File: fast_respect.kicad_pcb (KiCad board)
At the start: 2 copper layers, 70 x 110 mm, 97 parts, among them J1_1 Conn_02x04_Odd_Even, J5_1 Conn_02x03_Odd_Even, J5_2 Conn_02x03_Odd_Even, J7_1 Conn_01x02, Q2_1 AONM7421, Q3_1 IRLML6344T, Q4_1 IRLML6344T, Q4_2 IRLML6344T, Q4_3 IRLML6344T, Q4_4 IRLML6344T, Q4_5 ST-1KL3A, Q4_6 ST-1KL3A, Q4_7 ST-1KL3A, Q4_8 ST-1KL3A, Q7_1 IRLML6344T, SW1_1 BOOT0_SW, SW1_2 NRST_SW, SW2_1 SW_SPDT, SW3_1 SW_Push, SW3_2 SW_Push, SW3_3 SW_Push, U1_1 STM32F446RETx, U2_1 AZ1117-5.0, U2_2 AZ1117-3.3, U5_1 DRV8835DSSR, U6_1 ICM-42688-P

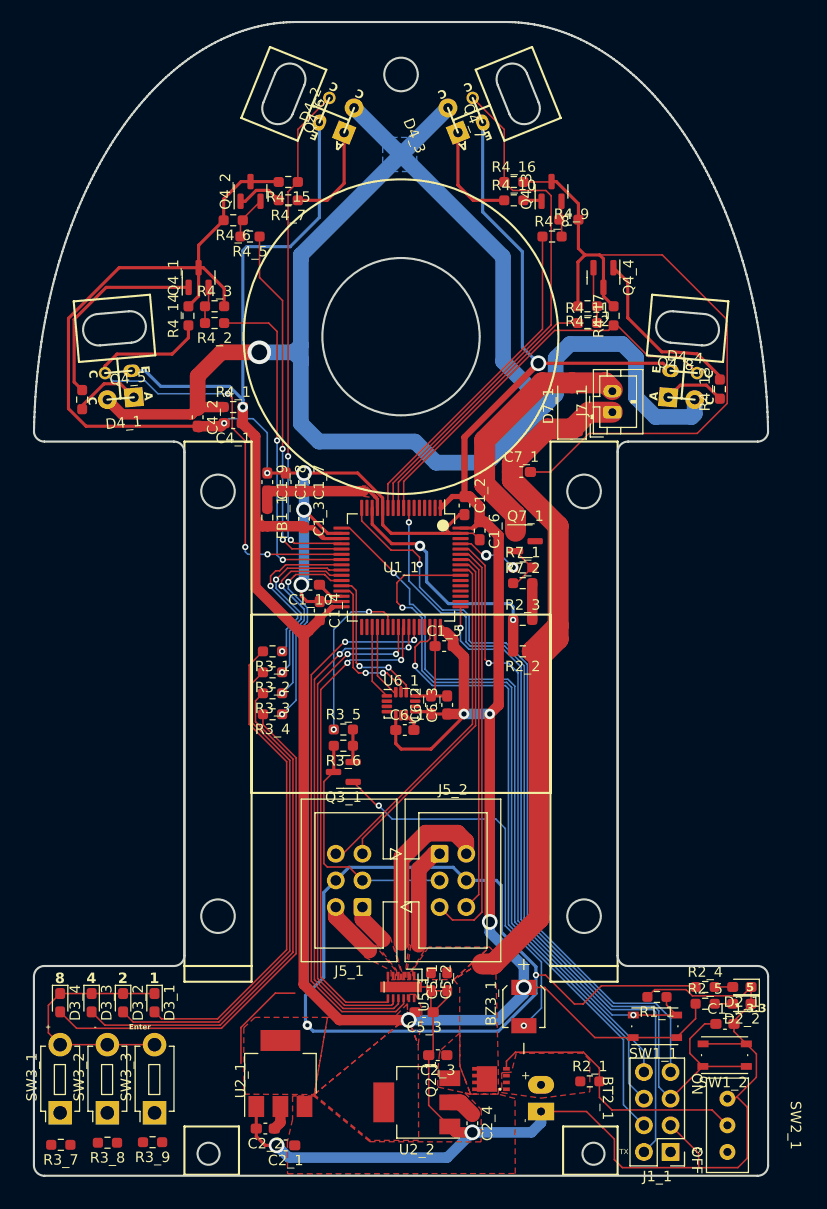
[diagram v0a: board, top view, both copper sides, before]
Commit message: UIスイッチ配線完了
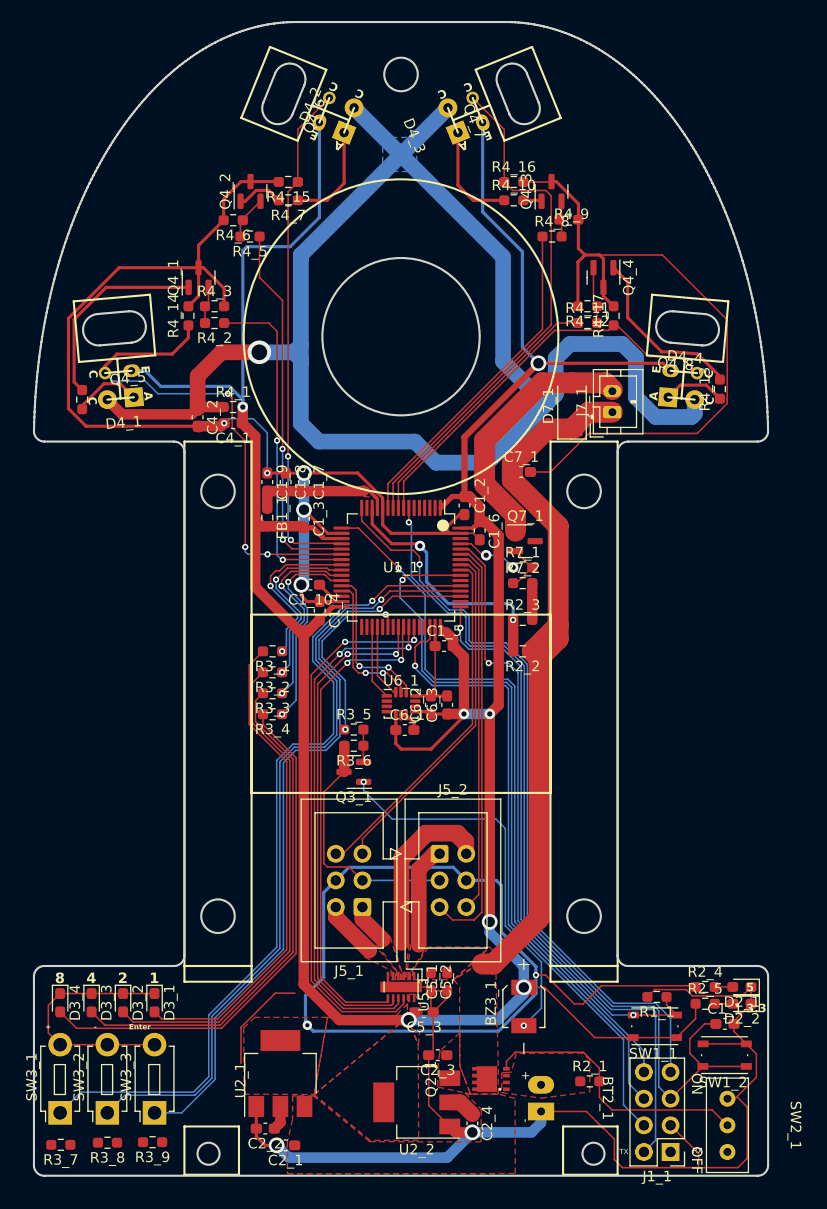
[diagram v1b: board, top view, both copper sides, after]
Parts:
- moved Q3_1 1.00 mm to (-39.5, 71.5)
- moved R3_5 1.00 mm to (-39.5, 67.5)
- moved R3_6 1.00 mm to (-39.5, 69.0)
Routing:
- net UI_SW_1: track 0.00 -> 81.1 mm, vias 0 -> 1
- net UI_SW_2: track 0.00 -> 76.4 mm, vias 0 -> 1
- net UI_SW_3: track 0.00 -> 71.7 mm, vias 0 -> 1
- net BUZZER_PWM: track 16.6 -> 17.7 mm
- net SWO: track 69.9 -> 69.0 mm
- net Net-(Q3_1-D): track 37.3 -> 36.7 mm
